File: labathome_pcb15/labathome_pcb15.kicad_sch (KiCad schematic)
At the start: 41 parts, among them J11 USB_ESP32, J15 CAN RS 485, J17 Micro_SD_Card_Det1, J21 GPIO, J22 Volts, J6 I2C, J7 PROG ESP, SW2 YELLOW, SW3 GREEN, SW3 Reset, SW4 RED, U2 ESP32-S3-WROOM-1, U21 IPS_240_240, U3 SRV05-4

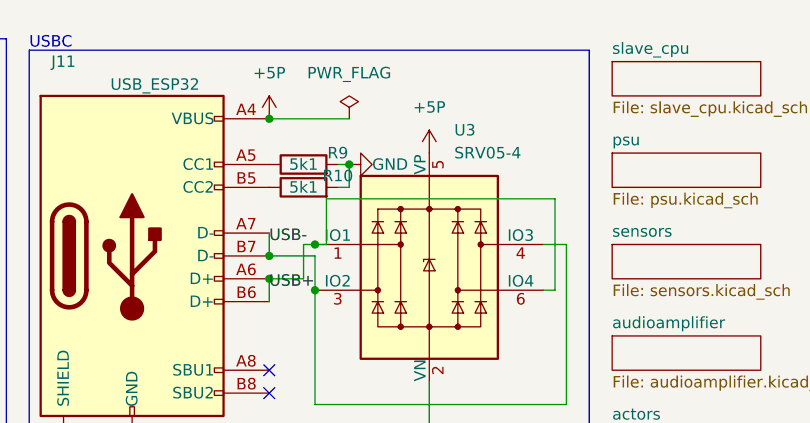
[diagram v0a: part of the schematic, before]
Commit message: IP5306
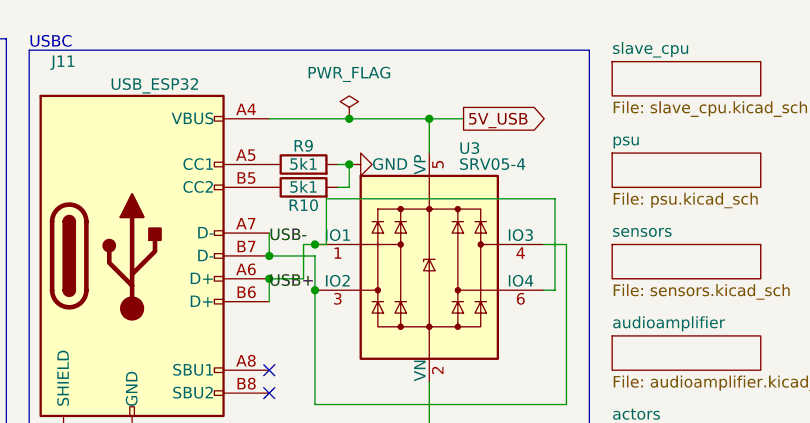
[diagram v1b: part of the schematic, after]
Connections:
- net +5P renamed 5V_USB
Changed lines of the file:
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@@
 	)
 	(junction
+		(at 212.09 22.86)
+		(diameter 0)
+		(color 0 0 0 0)
+	)
+	(junction
 		(at 16.51 82.55)
 		(diameter 0)
@@
 	)
 	(junction
-		(at 203.2 22.86)
-		(diameter 0)
-		(color 0 0 0 0)
-	)
-	(junction
 		(at 151.13 105.41)
 		(diameter 0)
@@
 	)
 	(junction
+		(at 220.98 22.86)
+		(diameter 0)
+		(color 0 0 0 0)
+	)
+	(junction
 		(at 27.94 110.49)
 		(diameter 0)
@@
 	(wire
 		(pts
+			(xy 220.98 22.86) (xy 212.09 22.86)
+		)
+		(stroke
+			(width 0)
+			(type default)
+		)
+	)
+	(wire
+		(pts
 			(xy 110.49 120.65) (xy 110.49 123.19)
 		)
@@
 	(wire
 		(pts
+			(xy 220.98 26.67) (xy 220.98 22.86)
+		)
+		(stroke
+			(width 0)
+			(type default)
+		)
+	)
+	(wire
+		(pts
 			(xy 210.82 27.94) (xy 212.09 27.94)
 		)
@@
 	(wire
 		(pts
+			(xy 220.98 22.86) (xy 224.79 22.86)
+		)
+		(stroke
+			(width 0)
+			(type default)
+		)
+	)
+	(wire
+		(pts
 			(xy 236.22 54.61) (xy 236.22 36.83)
 		)
@@
 		)
 	)
+	(global_label "5V_USB"
+		(shape output)
+		(at 224.79 22.86 0)
+		(fields_autoplaced yes)
+		(effects
+			(font
+				(size 1.27 1.27)
+			)
+			(justify left)
+		)
+		(property "Intersheetrefs" "${INTERSHEET_REFS}"
+			(at 234.8509 22.86 0)
+			(effects
+				(font
+					(size 1.27 1.27)
+				)
+				(justify left)
+				(hide yes)
+			)
+		)
+	)
 	(global_label "SDA"
 		(shape bidirectional)
@@
 		(on_board yes)
 		(dnp no)
-		(fields_autoplaced yes)
 		(property "Reference" "U3"
-			(at 223.7487 24.13 0)
+			(at 224.282 26.162 0)
 			(effects
 				(font
@@
 		)
 		(property "Value" "SRV05-4"
-			(at 223.7487 26.67 0)
+			(at 224.282 27.94 0)
 			(effects
 				(font
@@
 	)
 	(symbol
-		(lib_id "power:+5P")
-		(at 220.98 26.67 0)
-		(unit 1)
-		(exclude_from_sim no)
-		(in_bom yes)
-		(on_board yes)
-		(dnp no)
-		(fields_autoplaced yes)
-		(property "Reference" "#PWR054"
-			(at 220.98 30.48 0)
-			(effects
-				(font
-					(size 1.27 1.27)
-				)
-				(hide yes)
-			)
-		)
-		(property "Value" "+5P"
-			(at 220.98 21.59 0)
-			(effects
-				(font
-					(size 1.27 1.27)
-				)
-			)
-		)
-		(property "Footprint" ""
-			(at 220.98 26.67 0)
-			(effects
-				(font
-					(size 1.27 1.27)
-				)
-				(hide yes)
-			)
-		)
-		(property "Datasheet" ""
-			(at 220.98 26.67 0)
-			(effects
-				(font
-					(size 1.27 1.27)
-				)
-				(hide yes)
-			)
-		)
-		(property "Description" "Power symbol creates a global label with name \"+5P\""
-			(at 220.98 26.67 0)
-			(effects
-				(font
-					(size 1.27 1.27)
-				)
-				(hide yes)
-			)
-		)
-		(pin "1"
-		)
-		(instances
-			(project "labathome_pcb15"
-				(path "/e4d6926a-1a8b-424d-97c4-66b6ad87e4ac"
-					(reference "#PWR054")
-					(unit 1)
-				)
-			)
-		)
-	)
-	(symbol
 		(lib_id "Switch:SW_Push")
 		(at 17.78 44.45 90)
@@
 		(dnp no)
 		(property "Reference" "R9"
-			(at 210.82 26.67 90)
+			(at 207.01 25.908 90)
 			(effects
 				(font
@@
 		(dnp no)
 		(property "Reference" "R10"
-			(at 210.82 29.21 90)
+			(at 207.01 32.512 90)
 			(effects
 				(font
@@
 					(unit 1)
 				)
-			)
-		)
-	)
-	(symbol
-		(lib_id "power:+5P")
-		(at 203.2 22.86 0)
-		(unit 1)
-		(exclude_from_sim no)
-		(in_bom yes)
-		(on_board yes)
-		(dnp no)
-		(fields_autoplaced yes)
-		(property "Reference" "#PWR050"
-			(at 203.2 26.67 0)
-			(effects
-				(font
-					(size 1.27 1.27)
-				)
-				(hide yes)
-			)
-		)
-		(property "Value" "+5P"
-			(at 203.2 17.78 0)
-			(effects
-				(font
-					(size 1.27 1.27)
-				)
-			)
-		)
-		(property "Footprint" ""
-			(at 203.2 22.86 0)
-			(effects
-				(font
-					(size 1.27 1.27)
-				)
-				(hide yes)
-			)
-		)
-		(property "Datasheet" ""
-			(at 203.2 22.86 0)
-			(effects
-				(font
-					(size 1.27 1.27)
-				)
-				(hide yes)
-			)
-		)
-		(property "Description" "Power symbol creates a global label with name \"+5P\""
-			(at 203.2 22.86 0)
-			(effects
-				(font
-					(size 1.27 1.27)
-				)
-				(hide yes)
-			)
-		)
-		(pin "1"
-		)
-		(instances
-			(project "labathome_pcb15"
-				(path "/e4d6926a-1a8b-424d-97c4-66b6ad87e4ac"
-					(reference "#PWR050")
-					(unit 1)
-				)
